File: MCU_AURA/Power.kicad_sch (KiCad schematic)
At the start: 65 parts, among them J101 USB_C_Receptacle_USB2.0_16P, J3 XT30PW-M, U101 SI4825DDY-T1-GE3, U104 AP2127N-1.8, U2 TPS56C230RJER, U3 TPS2115ADRBR, U4 TLV62566DBVR

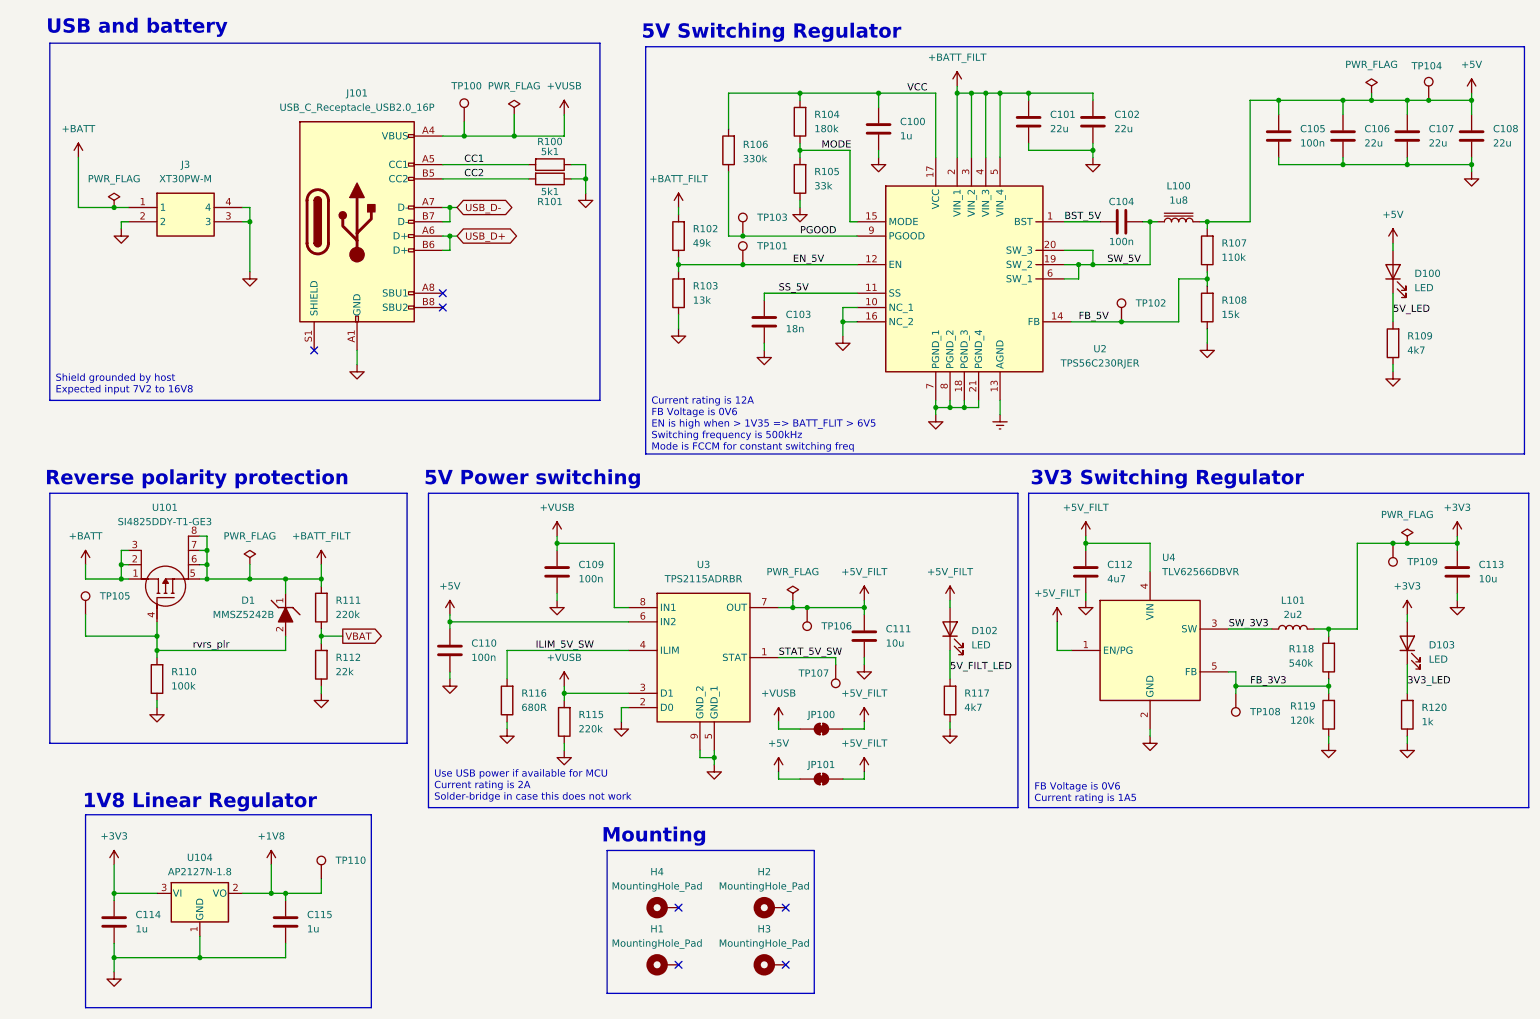
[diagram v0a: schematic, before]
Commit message: Initial Schematic Draft
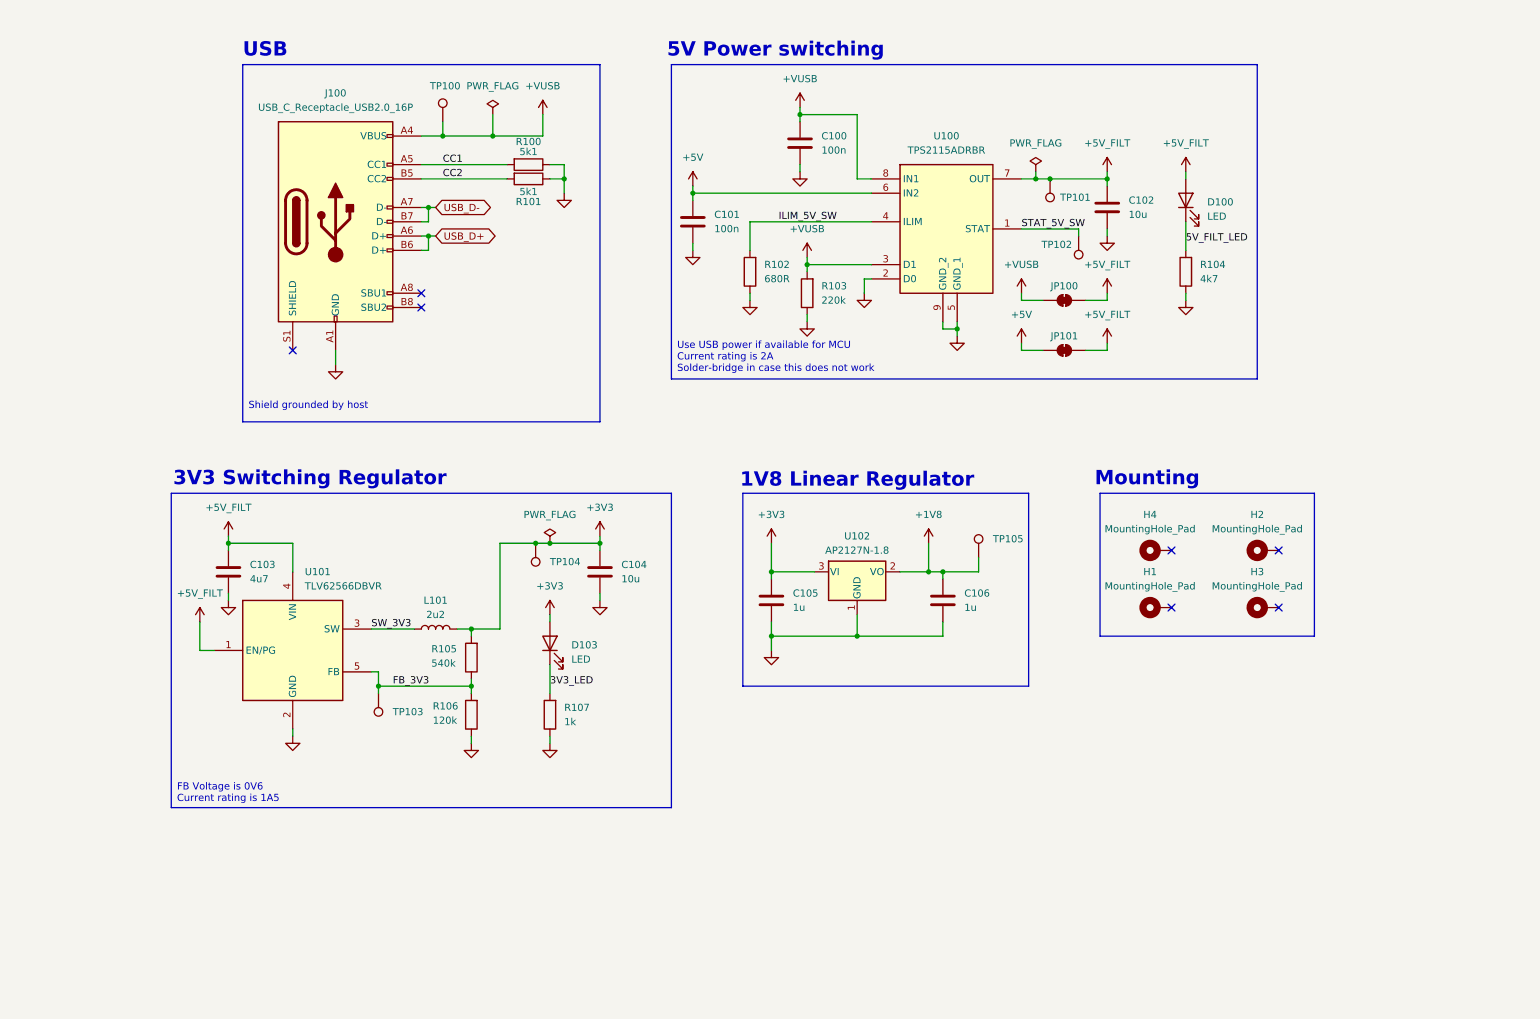
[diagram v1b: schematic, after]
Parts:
- removed C100: 1u, Capacitor_SMD:C_0402_1005Metric, symbol Device:C
- removed C101, C102: 22u, Capacitor_SMD:C_1206_3216Metric, symbol Device:C
- removed C103: 18n, Capacitor_SMD:C_0402_1005Metric, symbol Device:C
- removed C104: 100n, Capacitor_SMD:C_0402_1005Metric, symbol Device:C
- removed C105: 100n, Capacitor_SMD:C_0603_1608Metric, symbol Device:C
- removed C106, C107, C108: 22u, Capacitor_SMD:C_0805_2012Metric, symbol Device:C
- removed D1: MMSZ5242B, MMSZ5252B:MMSZ5252B, symbol MMSZ5252B:MMSZ5242B
- removed D100: LED, LED_SMD:LED_0603_1608Metric, symbol Device:LED
- removed J3: XT30PW-M, XT30PWM:XT30PWM, symbol XT30PW-M:XT30PW-M
- removed L100: 1u8, CKST0603:CKST0603-1.5uHM, symbol Device:L_Iron
- removed R102: 49k, Resistor_SMD:R_0402_1005Metric, symbol Device:R
- removed R103: 13k, Resistor_SMD:R_0402_1005Metric, symbol Device:R
- removed R104: 180k, Resistor_SMD:R_0402_1005Metric, symbol Device:R
- removed R105: 33k, Resistor_SMD:R_0402_1005Metric, symbol Device:R
- removed R106: 330k, Resistor_SMD:R_0402_1005Metric, symbol Device:R
- removed R107: 110k, Resistor_SMD:R_0402_1005Metric, symbol Device:R
- removed R108: 15k, Resistor_SMD:R_0402_1005Metric, symbol Device:R
- removed R109: 4k7, Resistor_SMD:R_0402_1005Metric, symbol Device:R
- removed R110: 100k, Resistor_SMD:R_0402_1005Metric, symbol Device:R
- removed R111: 220k, Resistor_SMD:R_0402_1005Metric, symbol Device:R
- removed R112: 22k, Resistor_SMD:R_0402_1005Metric, symbol Device:R
- removed TP101, TP102, TP103, TP104, TP105: TestPoint, TestPoint:TestPoint_Pad_D1.0mm, symbol Connector:TestPoint
- removed U101: SI4825DDY-T1-GE3, SI4825DDY-T1-GE3:SI4825DDY-T1-GE3, symbol SI4825DDY-T1-GE3:SI4825DDY-T1-GE3
- removed U2: TPS56C230RJER, TPS56C230RJER:QFN45P300X300X100-21N-D, symbol TPS56C230RJER:TPS56C230RJER
- renumbered C109 to C100, C110 to C101, C111 to C102, C112 to C103, C113 to C104, C114 to C105, C115 to C106, D102 to D100, J101 to J100, R116 to R102, R115 to R103, R117 to R104, R118 to R105, R119 to R106, R120 to R107, TP106 to TP101, TP107 to TP102, TP108 to TP103, TP109 to TP104, TP110 to TP105, U3 to U100, U4 to U101, U104 to U102
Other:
- note added: "Shield grounded by host"
- note added: "USB"
- note removed: "5V Switching Regulator"
- note removed: "Current rating is 12A FB Voltage is 0V6 EN is high when > 1V35 => BATT_FLIT > 6V5 Switching frequency is 500kHz Mode is FCCM for constant switching freq"
- note removed: "Reverse polarity protection"
- note removed: "Shield grounded by host Expected input 7V2 to 16V8"
- note removed: "USB and battery"
- moved on the sheet: C100, C101, C102, C103, C104, C105, C106, D100, D103, H1, H2, H3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

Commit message: Started Routing
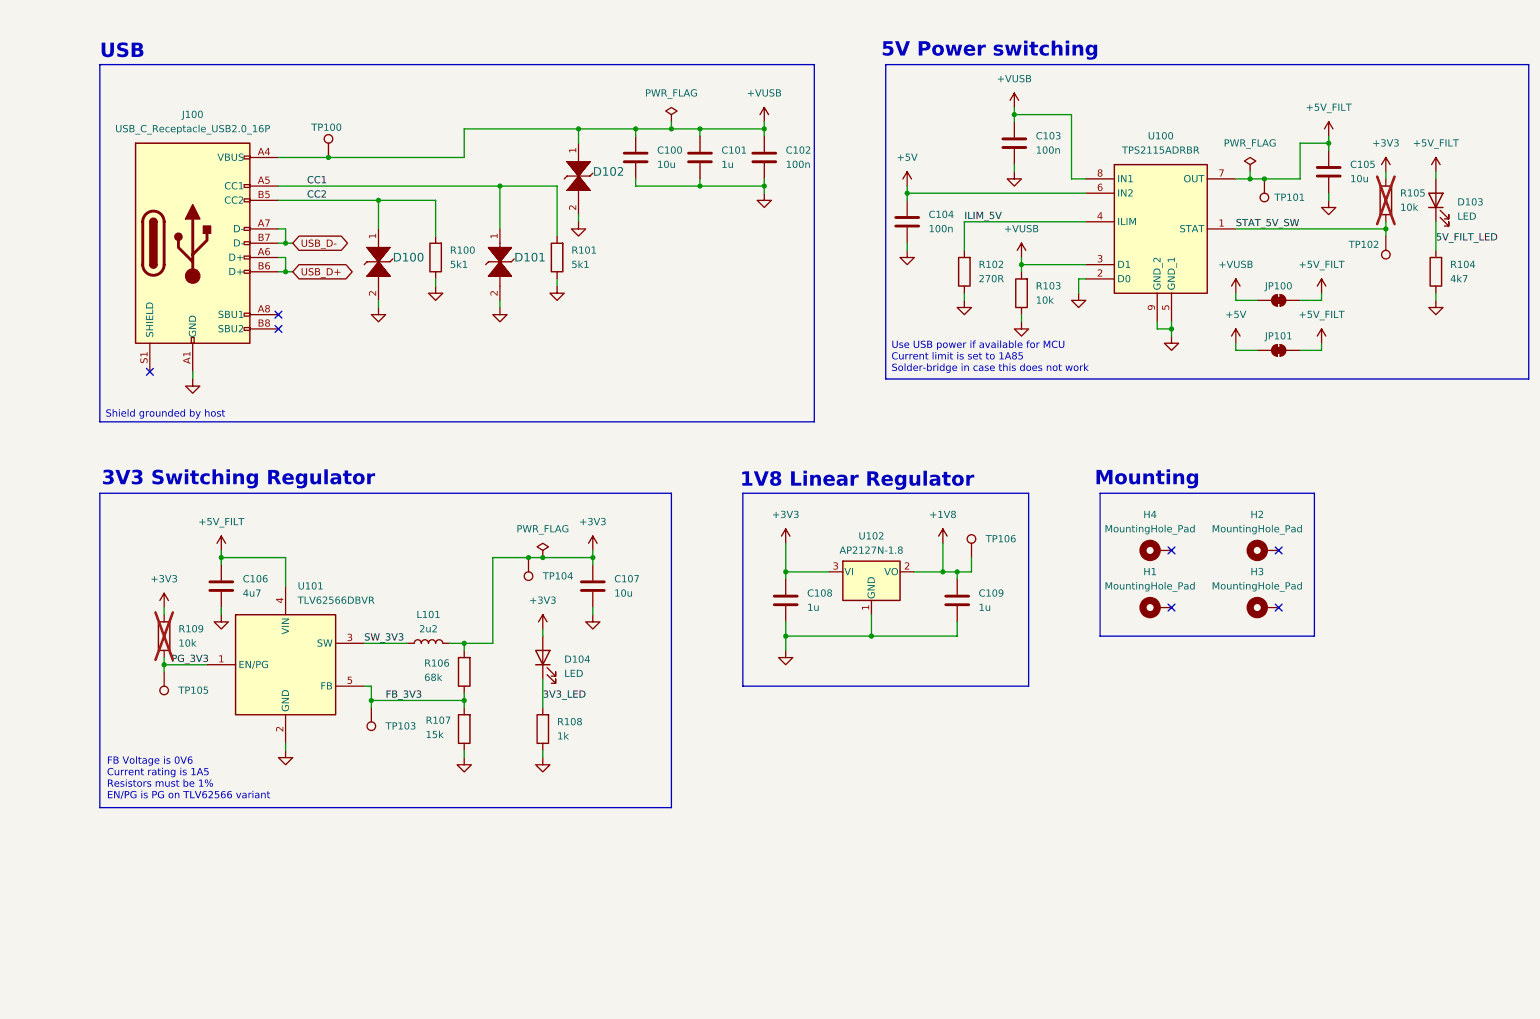
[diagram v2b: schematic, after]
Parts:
- added C100: 10u, Capacitor_SMD:C_0402_1005Metric, symbol Device:C
- added C101: 1u, Capacitor_SMD:C_0402_1005Metric, symbol Device:C
- added C102: 100n, Capacitor_SMD:C_0402_1005Metric, symbol Device:C
- added D100, D101, D102: TPD1E05U06DPYR, TPD1E05U06DPYR:DIO_TPD1E05U06DPYR, symbol ESDALC5_1BM2:ESDALC5-1BM2
- added R105, R109: 10k, Resistor_SMD:R_0402_1005Metric, symbol Device:R
- added TP105: TestPoint, TestPoint:TestPoint_Pad_D1.0mm, symbol Connector:TestPoint
- H1, H2, H3, H4: footprint MountingHole:MountingHole_4mm_Pad_Via -> MountingHole:MountingHole_3.2mm_M3_Pad_Via
- R102: value 680R -> 270R
- R103: value 220k -> 10k
- R106: renamed from R105; value 540k -> 68k
- R107: renamed from R106; value 120k -> 15k
- renumbered C100 to C103, C101 to C104, C102 to C105, C103 to C106, C104 to C107, C105 to C108, C106 to C109, D100 to D103, D103 to D104, R107 to R108, TP105 to TP106
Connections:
- net +3V3: now also R105.2, R109.2
- net +5V_FILT: no longer U101.1 (EN/PG)
- net +VUSB: now also C100.1, C101.1, C102.1, D102.1
- net CC1: now also R101.2, D101.1; no longer R100.2
- net CC2: now also R100.2, D100.1; no longer R101.2
- net GND: now also C100.2, C101.2, C102.2, D100.2, D101.2, D102.2
- net STAT_5V_SW: now also R105.1
- net ILIM_5V_SW renamed ILIM_5V
- new net PG_3V3: R109.1, TP105.1, U101.1 (EN/PG)
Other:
- note added: "FB Voltage is 0V6 Current rating is 1A5 Resistors must be 1% EN/PG is PG on TLV62566 variant"
- note added: "Use USB power if available for MCU Current limit is set to 1A85 Solder-bridge in case this does not work"
- note removed: "FB Voltage is 0V6 Current rating is 1A5"
- note removed: "Use USB power if available for MCU Current rating is 2A Solder-bridge in case this does not work"
- moved on the sheet: C103, C104, C105, C106, C107, C108, C109, D103, D104, J100, JP100, JP101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
